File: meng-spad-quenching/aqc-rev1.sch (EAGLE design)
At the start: 133 parts, among them IC1 ADCMP582, IC2 NC7SV74K8X, IC3 LT3032-5, IC4 OPA342, IC5 OPA342, IC6 LTC1711, IC7 DS1100LU-20+, IC8 LT3032-15, J1 VIN_LOGIC, M1 BSS806N, Q1 MMBTH81, Q2 MMBTH81, Q3 MMBTH81, Q4 MMBTH81, Q5 MMBTH81, Q6 MMBTH81, T1 MMBTH10, T2 MMBTH10, T3 MMBTH10, T4 MMBTH10, T5 MMBTH10, T6 MMBTH10, T7 MMBTH10, U1 SN65EPT21DGK, U2 TPS78233DDCT, U3 SN65EPT22DGK, X1 CONN_SPAD, X2 CONN_SCOPE_COMP, X3 CONN_SCOPE_RSHUNT, X4 CONN_VREF_ONE_SHOT_EXT, X5 CONN_VREF_DIAMOND_IBIAS_EXT, X6 CONN_VREF_CASCODE_IBIAS_EXT

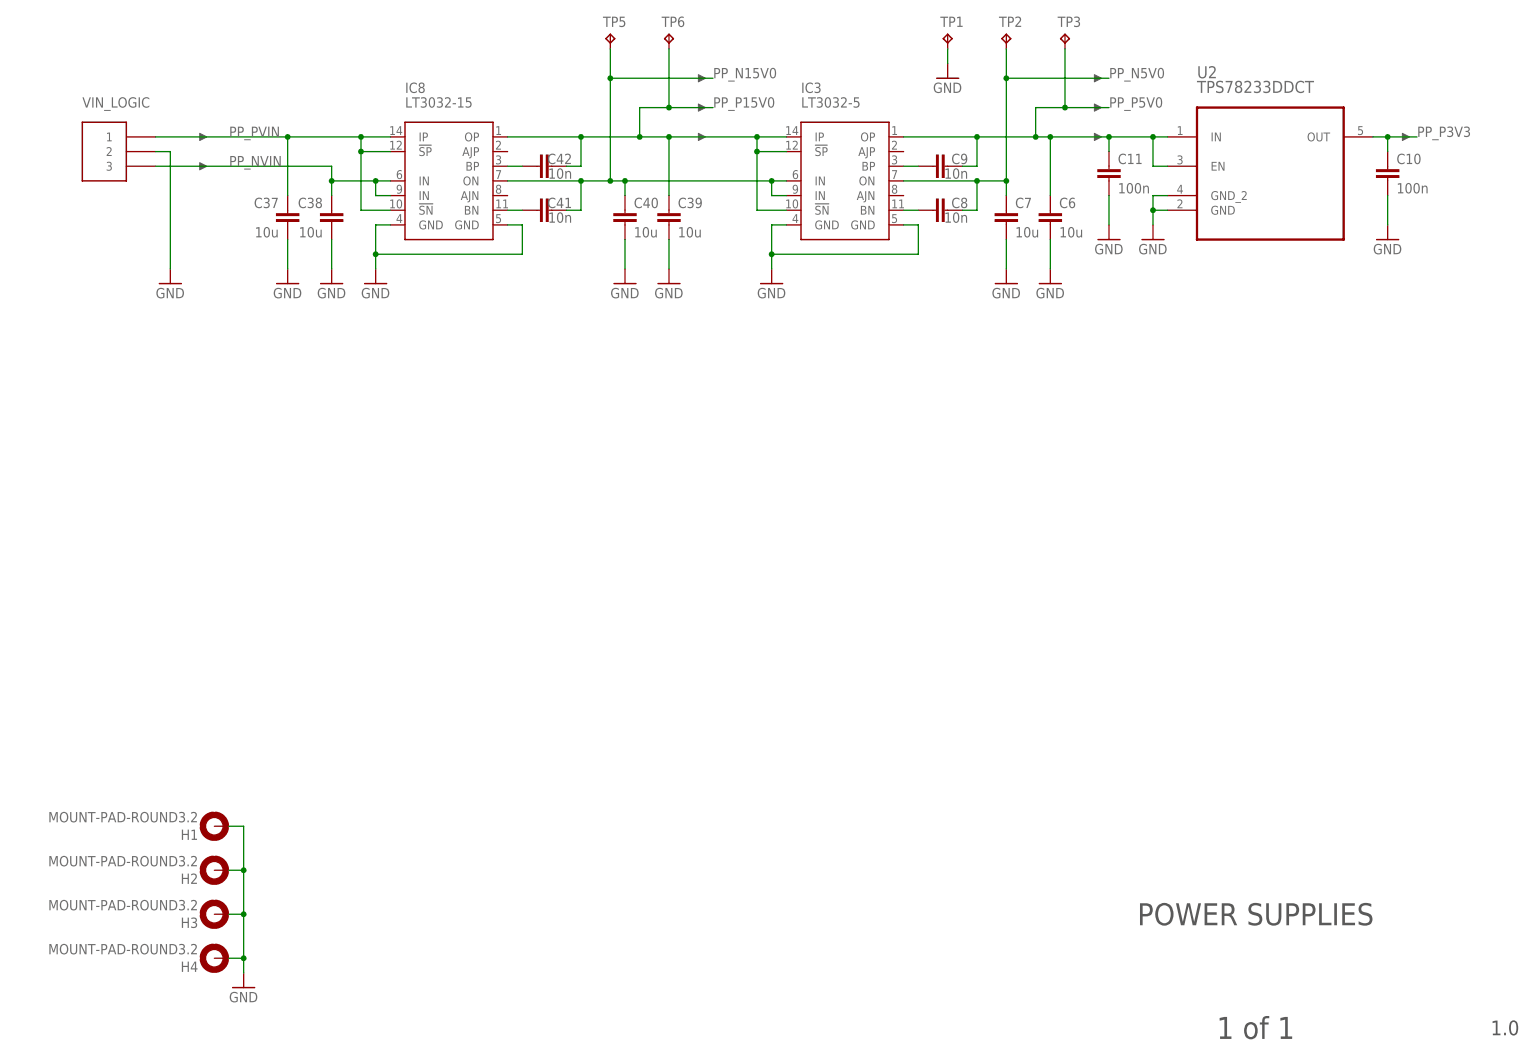
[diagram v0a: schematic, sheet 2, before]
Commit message: More routing
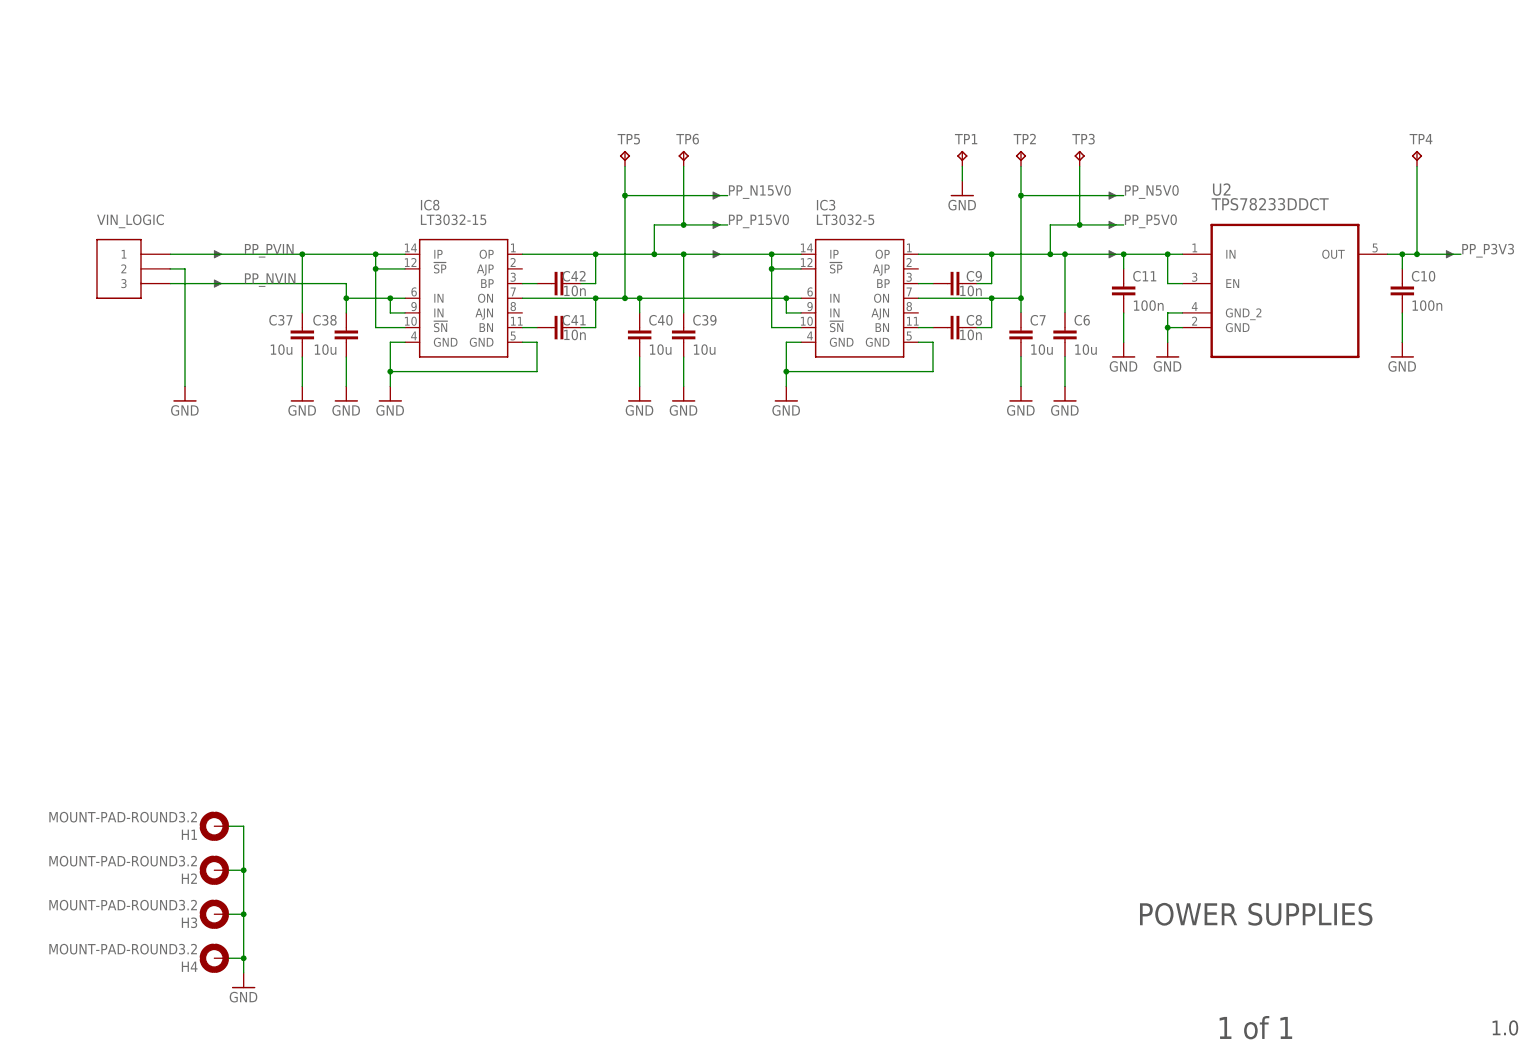
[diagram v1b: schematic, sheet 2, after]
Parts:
- removed R6: 49R9, rcl:R-EU_R0603
- removed X3: CONN_SCOPE_RSHUNT, con-coax:SMA-142-0711-871/876
- added C43: 10n, rcl:C-EUC0603
- added C44: 100n, rcl:C-EUC0603
- added IC9: NC7WZ16P6X, meng:NC7WZ16P6X
- added TP4: TPTP20R, testpad:TPTP20R
- R4: value DNP -> 49R9
- X2: value CONN_SCOPE_COMP -> CONN_PHOTON_COUNTER
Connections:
- removed net N$36: IC3.!SN, IC3.!SP, IC3.IP
- removed net VSCOPE_1: R4.2, X3G1.1
- new net N$35: IC5.-IN, R29.2, T7.E
- new net N$37: IC9.OUT1, IC9.OUT2, R4.2
- net GND: now also C43.2, C44.2, IC9.GND; no longer X3G1.GND
- net HOLDOFF_TRIG: no longer R6.2
- net LOGIC_QUENCH: now also IC9.IN1, IC9.IN2
- net N$2: now also R4.1; no longer R6.1
- net PP_N5V0: no longer IC5.-IN, R29.2, T7.E
- net PP_P15V0: now also IC3.!SN, IC3.!SP, IC3.IP
- net PP_P3V3: now also C43.1, C44.1, IC9.VCC, TP4.TP
- net SPAD_PULLDN_SENSE: no longer R4.1
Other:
- note added: "To pulse counter"
- note removed: "To scope"
- moved on the sheet: C10, C11, C37, C38, C39, C40, C41, C42, C6, C7, C8, C9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
